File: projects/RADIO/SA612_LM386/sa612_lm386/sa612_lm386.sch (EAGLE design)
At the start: 41 parts, among them IC1 SA612AN_01,112, IC2 LM386M-1, IC3 LM1117MPX-33NOPB, Q1 BF245

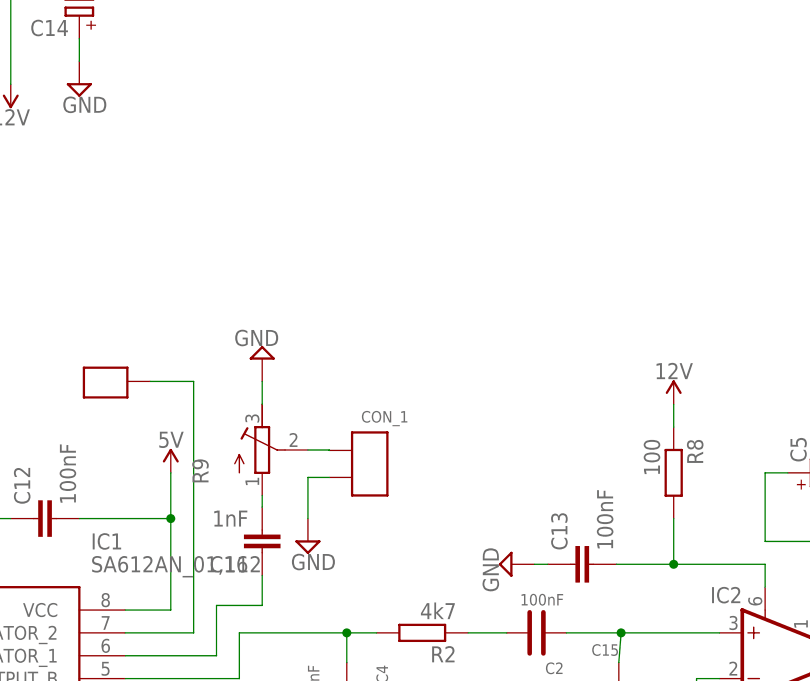
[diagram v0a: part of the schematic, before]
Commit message: update
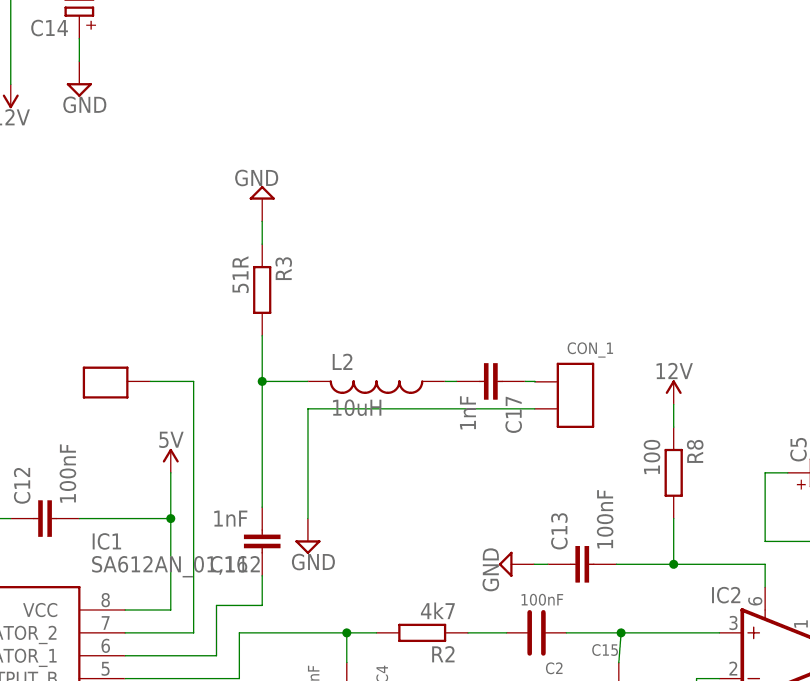
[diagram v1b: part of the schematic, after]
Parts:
- removed R9: (no value), rcl:R-TRIMM64W
- added C17: 1nF, mylib:C_0805_SMD
- added L2: 10uH, mylib:L_0805_PTH
- added R3: 51R, mylib:R_0805_SMD
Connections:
- new net N$23: C17.2, L2.1
- net GND: now also R3.1; no longer R9.E
- net N$22: now also C17.1; no longer R9.S
- net N$5: now also L2.2, R3.2; no longer R9.A
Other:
- moved on the sheet: CON_1
